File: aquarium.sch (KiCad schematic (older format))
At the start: 39 parts, among them U1 MOC3063, U2 MOC3063

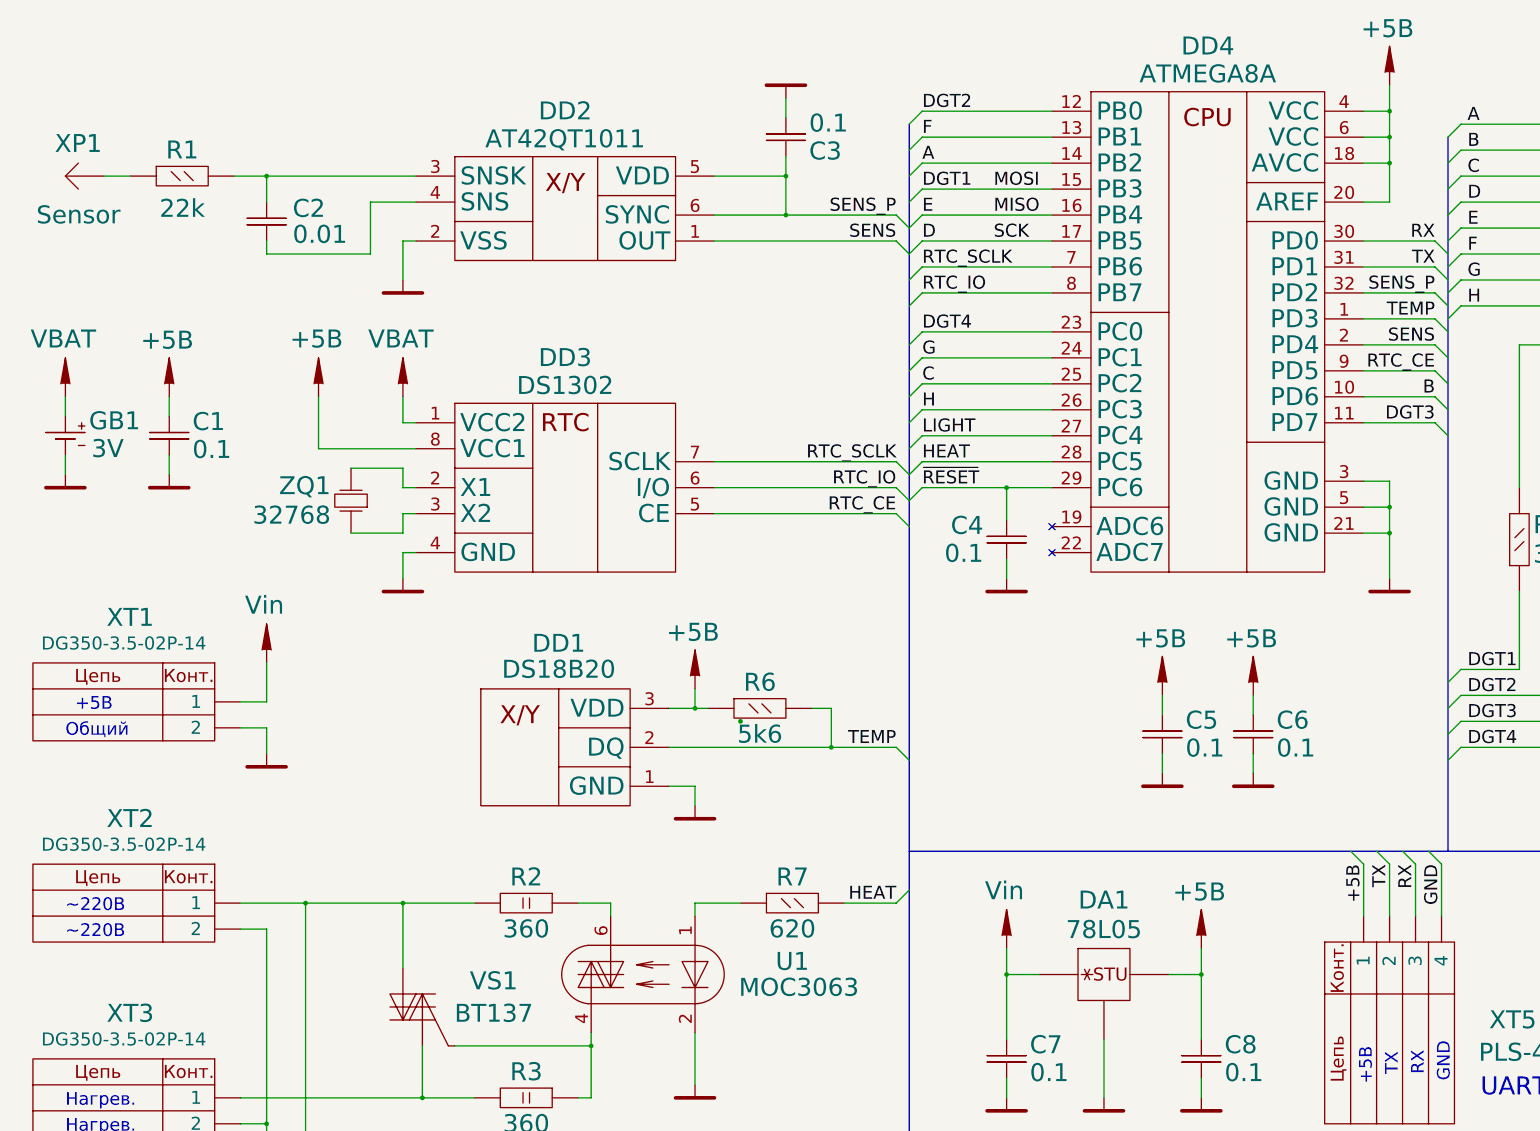
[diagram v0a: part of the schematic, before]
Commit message: Revert "Added possibility to calibrate the capacitive sensor."
This reverts commit 56735a840efcf7c901892eb1b50b215983c0ef84.
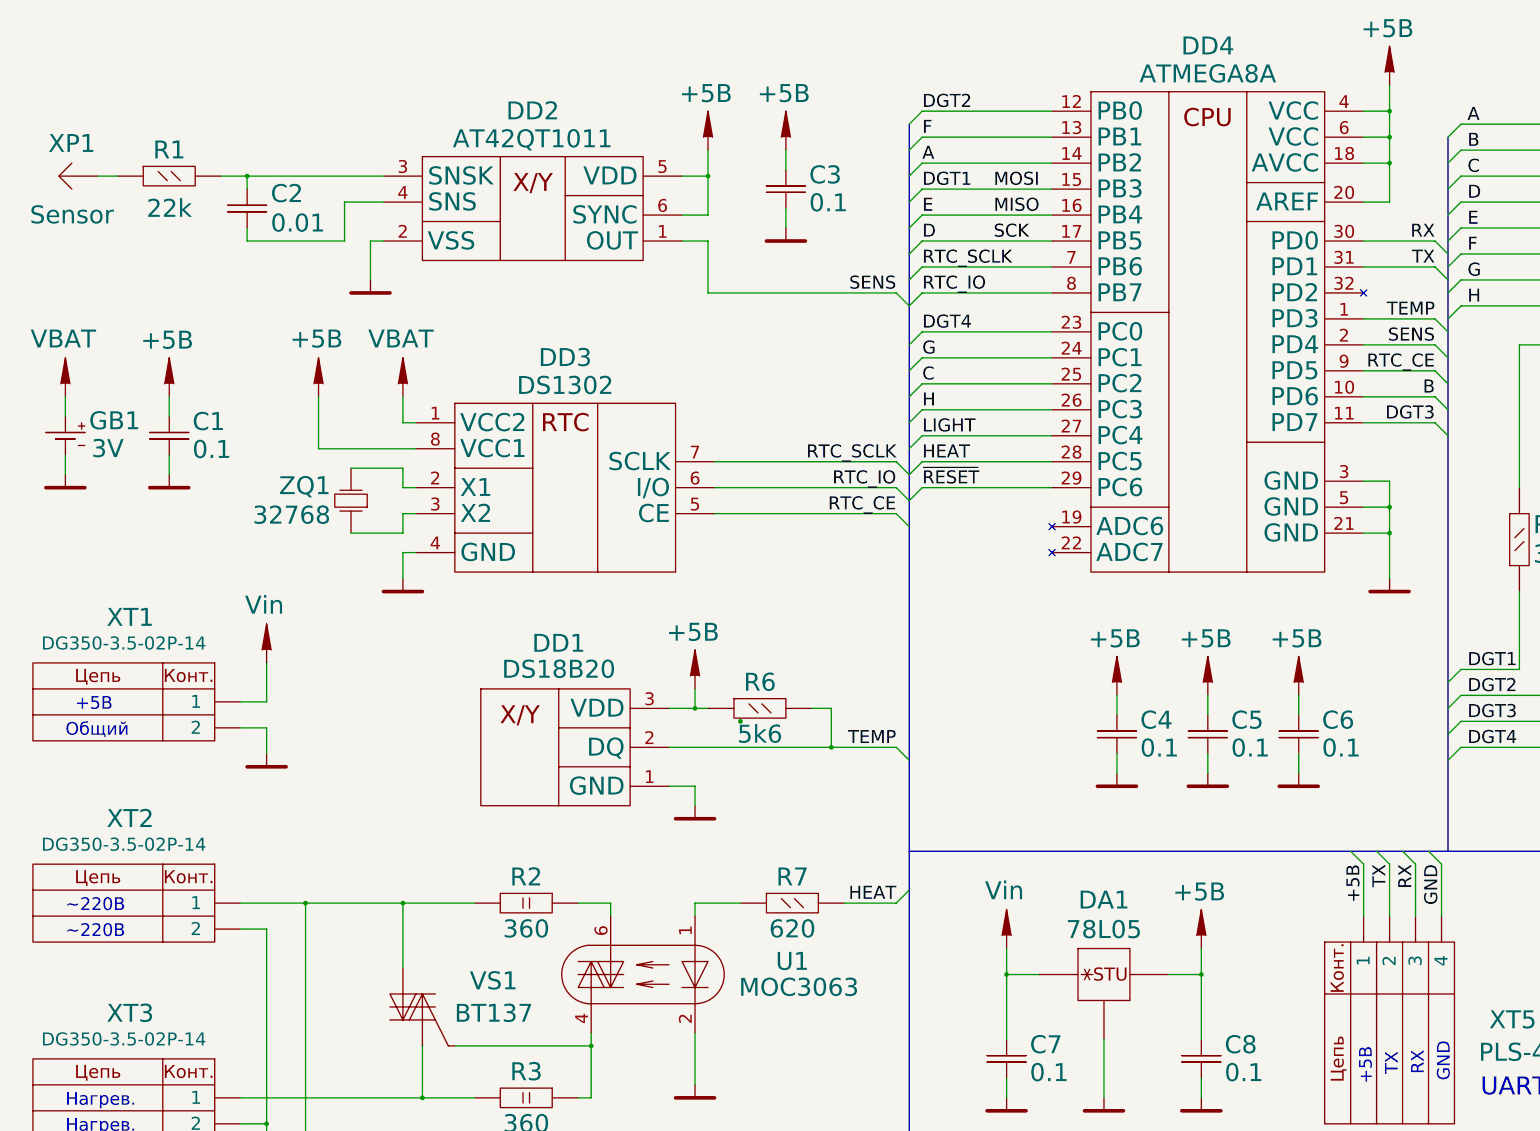
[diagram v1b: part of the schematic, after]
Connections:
- net +5B: now also C3.1, C4.1, DD2.5 (VDD), DD2.6 (SYNC)
- net ~RESET: no longer C4.1
- removed net SENS_P: C3.1, DD2.5 (VDD), DD2.6 (SYNC), DD4.32 (PD2)
- no-connect marks 2 -> 3
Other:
- moved on the sheet: C2, C3, C5, C6, DD2, R1, XP1

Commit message: Added possibility to calibrate the capacitive sensor.
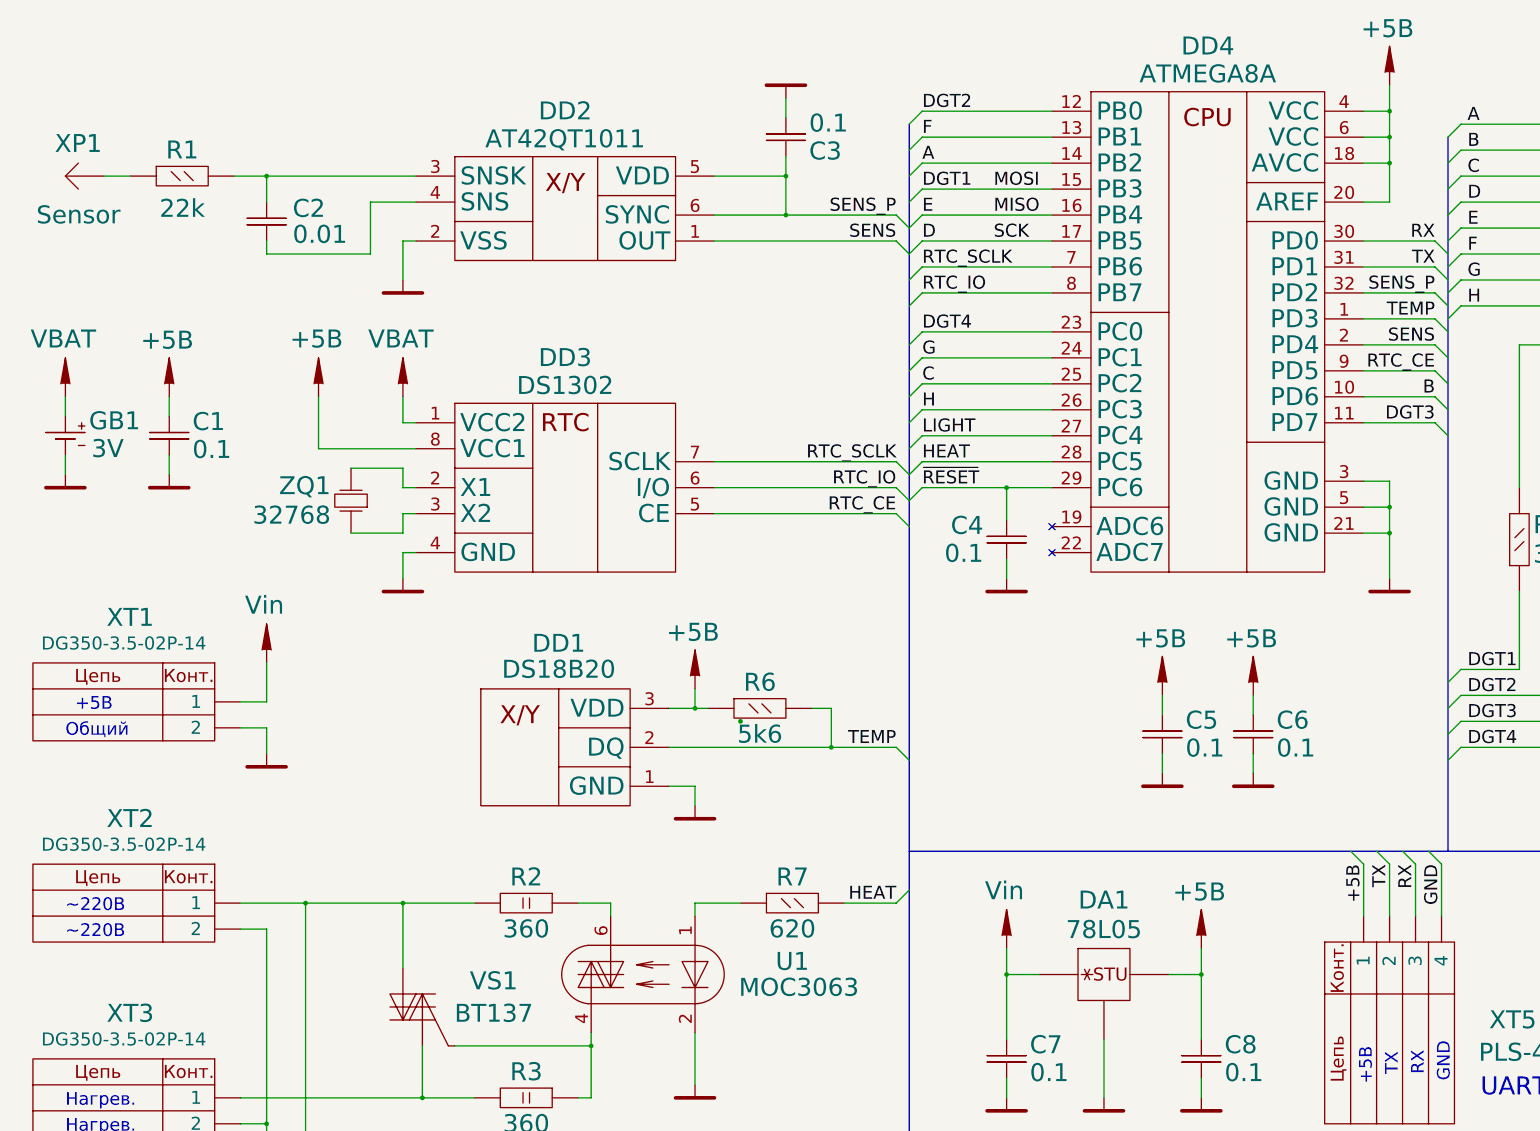
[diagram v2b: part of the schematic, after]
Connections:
- net +5B: no longer C3.1, C4.1, DD2.5 (VDD), DD2.6 (SYNC)
- net ~RESET: now also C4.1
- net SENS_P: now reaches DD4.32 (PD2)
- net SENS_P: now also C3.1, DD2.5 (VDD), DD2.6 (SYNC)
- no-connect marks 3 -> 2
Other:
- moved on the sheet: C2, C3, C5, C6, DD2, R1, XP1
